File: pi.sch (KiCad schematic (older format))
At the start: 26 parts, among them T2 QT24A01, U1 rpi_cm4, U2 m.2_pcie_nvme

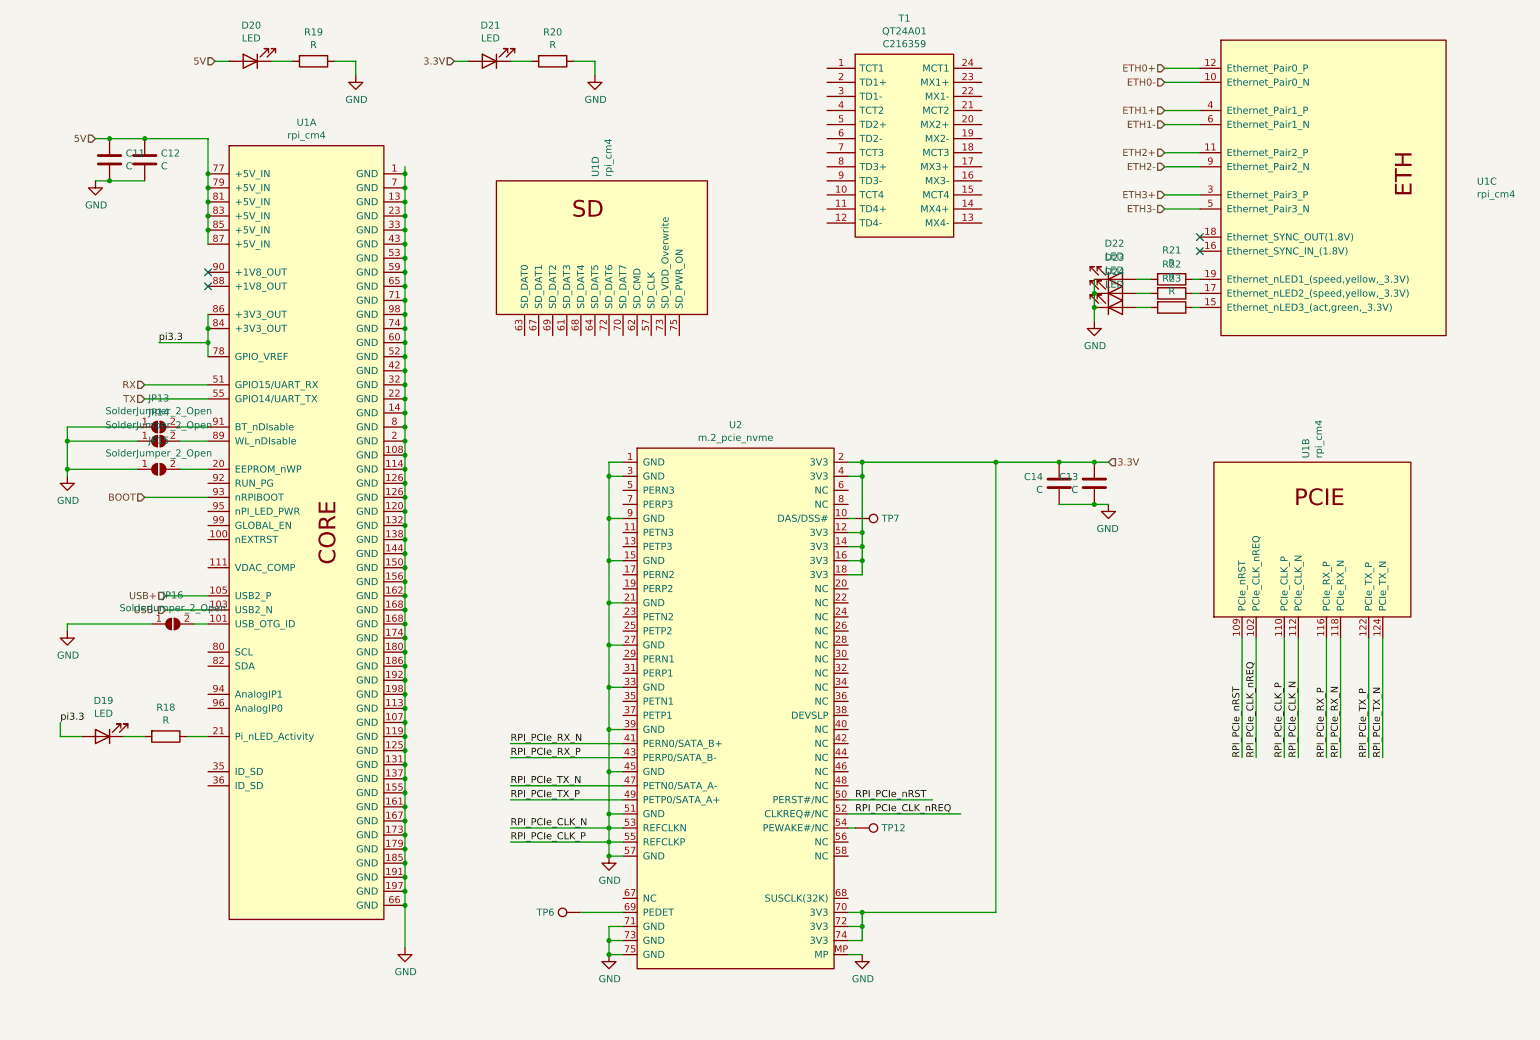
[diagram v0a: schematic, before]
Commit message: Organized pi.sch document.
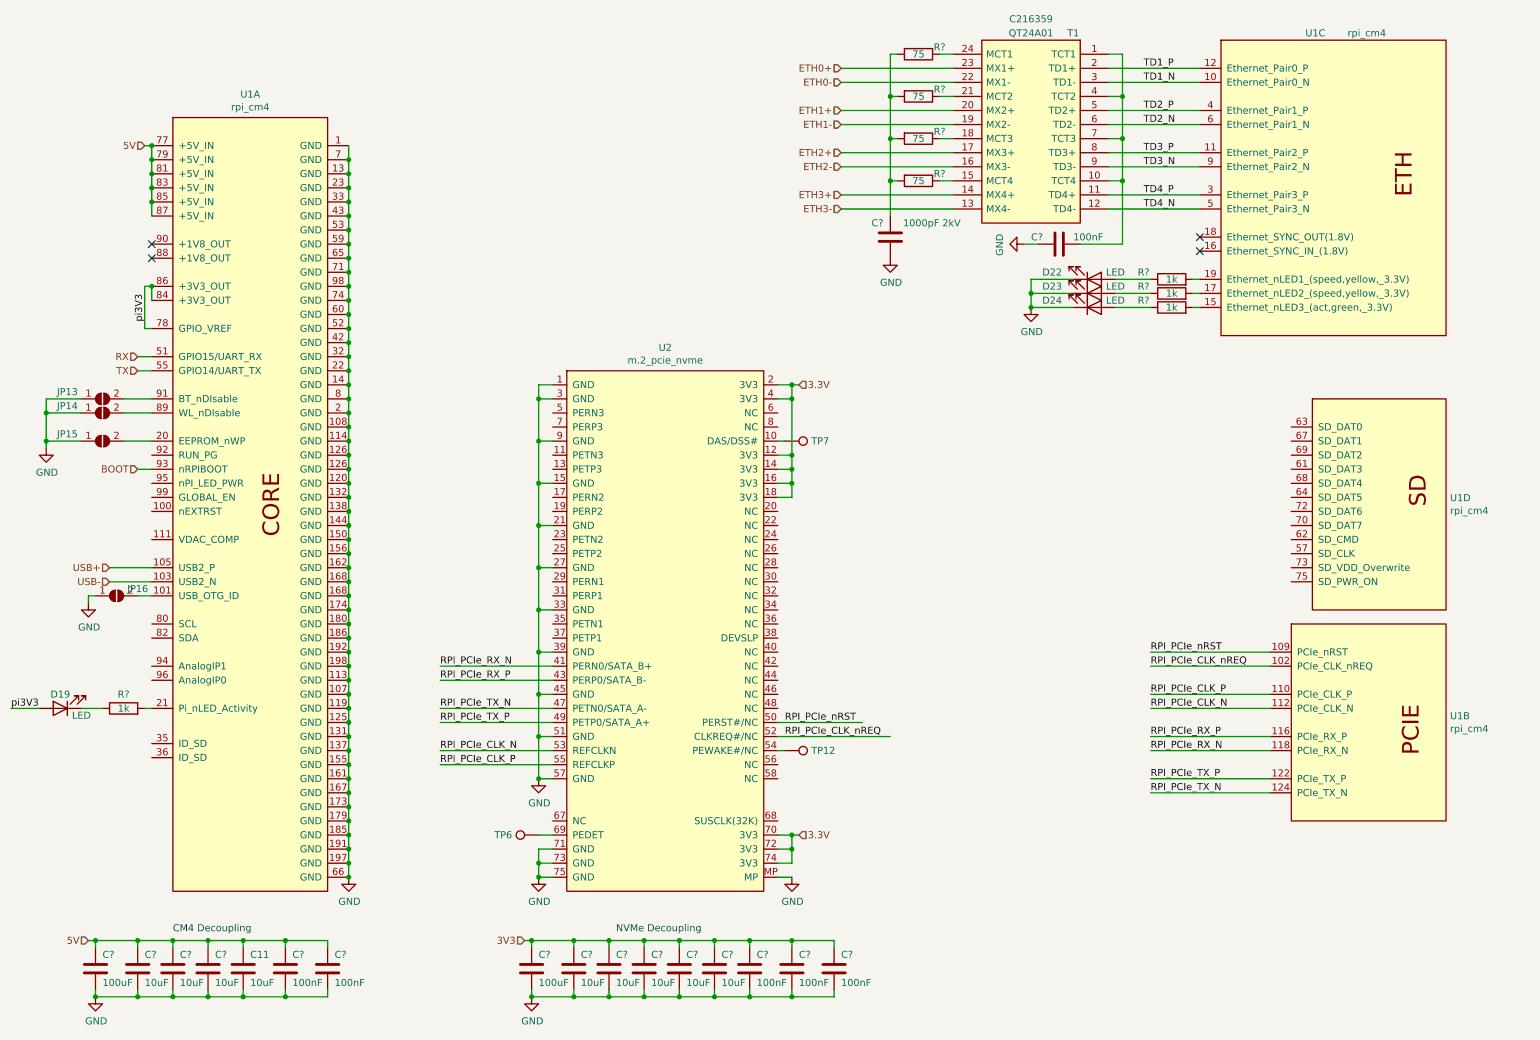
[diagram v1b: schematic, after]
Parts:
- removed C2, C4: C, Capacitor_SMD:C_0603_1608Metric, symbol Device:C
- removed C3: C, Capacitor_SMD:C_0805_2012Metric, symbol Device:C
- removed D3, D4: LED, LED_SMD:LED_0603_1608Metric, symbol Device:LED
- removed R1, R2, R3, R4, R5, R6: R, Resistor_SMD:R_0603_1608Metric, symbol Device:R
- added C? (x8): 10uF, Capacitor_SMD:C_0805_2012Metric, symbol Device:C
- added C? (x2): 100uF, Capacitor_SMD:C_1206_3216Metric, symbol Device:C
- added C? (x6): 100nF, Capacitor_SMD:C_0402_1005Metric, symbol Device:C
- added C?: 1000pF 2kV, Capacitor_SMD:C_1206_3216Metric, symbol Device:C
- added R? (x4): 1k, Resistor_SMD:R_0402_1005Metric, symbol Device:R
- added R? (x4): 75, Resistor_SMD:R_0402_1005Metric, symbol Device:R
- C1: value C -> 10uF
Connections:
- net 5V: now also C?.1, C?.1, C?.1, C?.1, C?.1, C?.1
- net ETH0+: now also T2.23 (MX1+); no longer U1.12 (Ethernet_Pair0_P)
- net ETH0-: now also T2.22 (MX1-); no longer U1.10 (Ethernet_Pair0_N)
- net ETH1+: now also T2.20 (MX2+); no longer U1.4 (Ethernet_Pair1_P)
- net ETH1-: now also T2.19 (MX2-); no longer U1.6 (Ethernet_Pair1_N)
- net ETH2+: now also T2.17 (MX3+); no longer U1.11 (Ethernet_Pair2_P)
- net ETH2-: now also T2.16 (MX3-); no longer U1.9 (Ethernet_Pair2_N)
- net ETH3+: now also T2.14 (MX4+); no longer U1.3 (Ethernet_Pair3_P)
- net ETH3-: now also T2.13 (MX4-); no longer U1.5 (Ethernet_Pair3_N)
- net GND: now also C?.1, C?.2, C?.2, C?.2, C?.2, C?.2, C?.2, C?.2, C?.2, C?.2, C?.2, C?.2, C?.2, C?.2, C?.2, C?.2, C?.2; no longer U1.110 (PCIe_CLK_P), U1.112 (PCIe_CLK_N), U2.53 (REFCLKN), U2.55 (REFCLKP)
- net at U1.21 (Pi_nLED_Activity): now also R?.2
- net at U1.15 (Ethernet_nLED3_(act,green,_3.3V)): now also R?.2
- net at U1.17 (Ethernet_nLED2_(speed,yellow,_3.3V)): now also R?.2
- net at U1.19 (Ethernet_nLED1_(speed,yellow,_3.3V)): now also R?.2
- net at D2.1 (K): now also R?.1
- net at D5.2 (A): now also R?.1
- net at D6.2 (A): now also R?.1
- net at D7.2 (A): now also R?.1
- net at T2.1 (TCT1): now also T2.10 (TCT4), T2.4 (TCT2), T2.7 (TCT3), C?.1
- net TD4_P: now reaches T2.11 (TD4+)
- net TD4_P: now also U1.3 (Ethernet_Pair3_P)
- net TD4_N: now reaches T2.12 (TD4-)
- net TD4_N: now also U1.5 (Ethernet_Pair3_N)
- net at T2.15 (MCT4): now also R?.1
- net at T2.18 (MCT3): now also R?.1
- net TD1_P: now reaches T2.2 (TD1+)
- net TD1_P: now also U1.12 (Ethernet_Pair0_P)
- net at T2.21 (MCT2): now also R?.1
- net at T2.24 (MCT1): now also R?.1
- net TD1_N: now reaches T2.3 (TD1-)
- net TD1_N: now also U1.10 (Ethernet_Pair0_N)
- net TD2_P: now reaches T2.5 (TD2+)
- net TD2_P: now also U1.4 (Ethernet_Pair1_P)
- net TD2_N: now reaches T2.6 (TD2-)
- net TD2_N: now also U1.6 (Ethernet_Pair1_N)
- net TD3_P: now reaches T2.8 (TD3+)
- net TD3_P: now also U1.11 (Ethernet_Pair2_P)
- net TD3_N: now reaches T2.9 (TD3-)
- net TD3_N: now also U1.9 (Ethernet_Pair2_N)
- net pi3.3 renamed pi3V3
- new net: C?.2, R?.2, R?.2, R?.2, R?.2
- new net 3V3: C?.1, C?.1, C?.1, C?.1, C?.1, C?.1, C?.1, C?.1, C?.1
- new net RPI_PCIe_CLK_N: U1.112 (PCIe_CLK_N), U2.53 (REFCLKN)
- new net RPI_PCIe_CLK_P: U1.110 (PCIe_CLK_P), U2.55 (REFCLKP)
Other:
- note added: "CM4 Decoupling"
- note added: "NVMe Decoupling"
- moved on the sheet: C11, D19, D22, D23, D24, JP13, JP14, JP15, JP16, T1, TP12, TP6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
